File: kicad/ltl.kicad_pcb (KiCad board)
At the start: 2 copper layers, 73 x 46 mm, 14 parts, among them J1 Serial Connection, J2 BARREL_JACK, SW1 SW_DIP_x02, SW2 SW_DIP_x02, U1 ESP-12E, U2 DS18B20

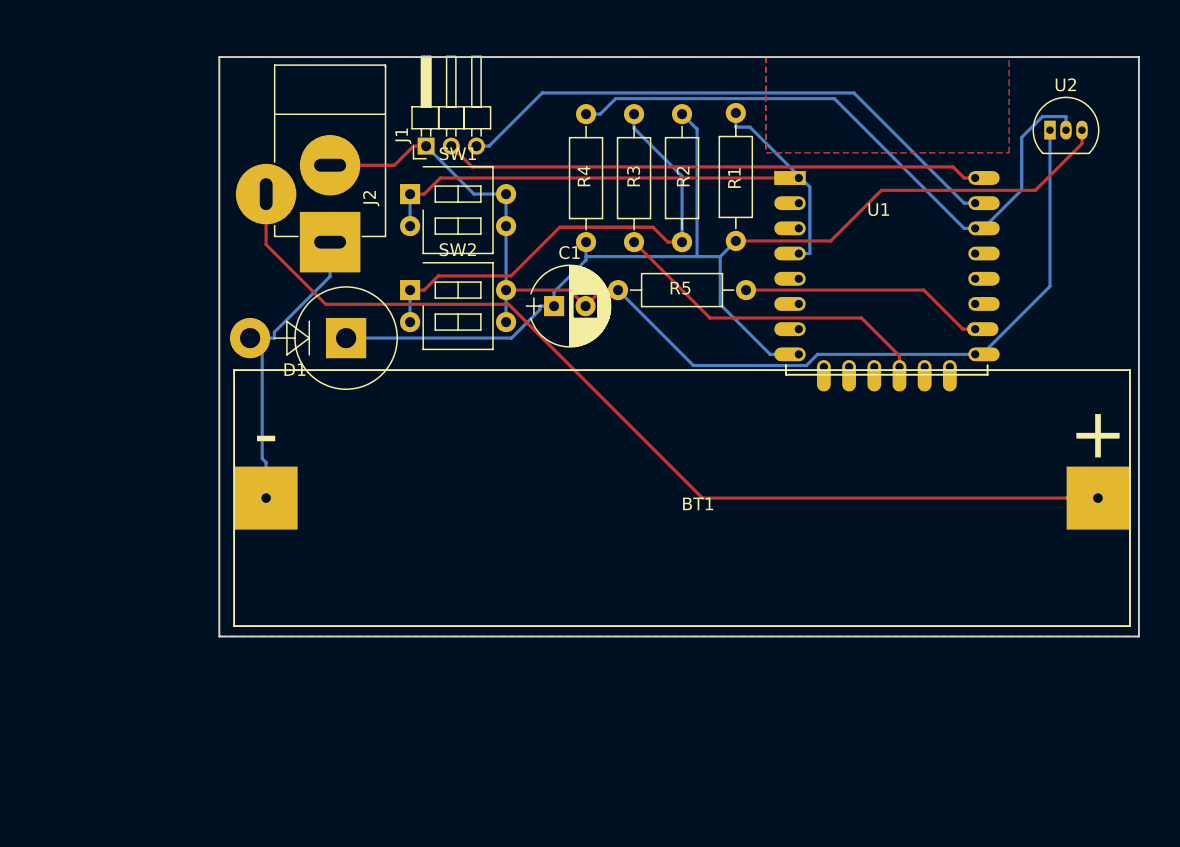
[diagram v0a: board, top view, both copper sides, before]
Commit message: letzte Änderungen
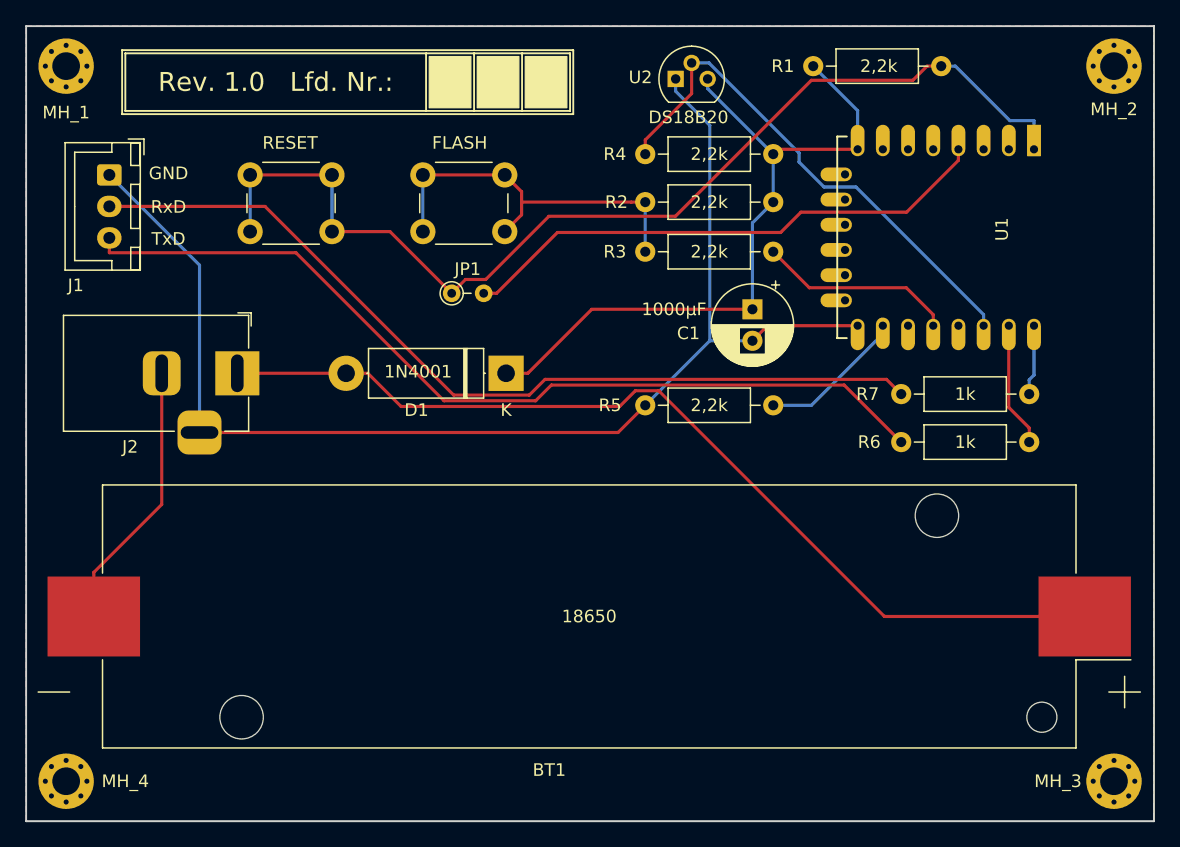
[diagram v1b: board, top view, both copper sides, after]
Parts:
- removed SW1, SW2: SW_DIP_x02, Buttons_Switches_THT:SW_DIP_x2_W7.62mm_Slide_LowProfile
- added FLASH: SW_DIP_x02, Button_Switch_THT:SW_PUSH_6mm_H5mm, F.Cu at (105.2, 79.8)
- added JP1: Jumper, Resistor_THT:R_Axial_DIN0204_L3.6mm_D1.6mm_P2.54mm_Vertical, F.Cu at (107.4, 89.2)
- added MH_1: MH_1, MountingHole:MountingHole_2.2mm_M2_Pad_Via, F.Cu at (76.8, 71.1)
- added MH_2: MH_2, MountingHole:MountingHole_2.2mm_M2_Pad_Via, F.Cu at (160.0, 71.1)
- added MH_3: MH_3, MountingHole:MountingHole_2.2mm_M2_Pad_Via, F.Cu at (160.0, 127.9)
- added MH_4: MH_4, MountingHole:MountingHole_2.2mm_M2_Pad_Via, F.Cu at (76.8, 127.9)
- added R6: 1k, Resistor_THT:R_Axial_DIN0207_L6.3mm_D2.5mm_P10.16mm_Horizontal, F.Cu at (143.1, 101.0)
- added R7: 1k, Resistor_THT:R_Axial_DIN0207_L6.3mm_D2.5mm_P10.16mm_Horizontal, F.Cu at (143.1, 97.2)
- added RESET: SW_DIP_x02, Button_Switch_THT:SW_PUSH_6mm_H5mm, F.Cu at (91.4, 79.8)
- BT1: footprint 18650:18650 -> Battery:BatteryHolder_Keystone_1042_1x18650
- C1: footprint Capacitors_THT:CP_Radial_D6.3mm_P2.50mm -> Capacitor_THT:CP_Radial_D6.3mm_P2.50mm
- D1: value D -> 1N4001; footprint Diodes_THT:D_5KPW_P7.62mm_Vertical_AnodeUp -> Diode_THT:D_5W_P12.70mm_Horizontal
- J1: value Serial Connection -> CONN_01X03; footprint Pin_Headers:Pin_Header_Angled_1x03_Pitch2.00mm -> Connector_JST:JST_XH_B3B-XH-A_1x03_P2.50mm_Vertical
- J2: footprint Connectors:JACK_ALIM -> Connector_BarrelJack:BarrelJack_Horizontal
- R1, R2, R3, R4, R5: footprint Resistors_THT:R_Axial_DIN0207_L6.3mm_D2.5mm_P10.16mm_Horizontal -> Resistor_THT:R_Axial_DIN0207_L6.3mm_D2.5mm_P10.16mm_Horizontal
- U2: footprint TO_SOT_Packages_THT:TO-92_Inline_Narrow_Oval -> Package_TO_SOT_THT:TO-92
- moved U2 30.0 mm to (125.2, 72.1)
- moved J1 25.2 mm to (80.3, 79.8), turned to 270 degrees
- moved U1 18.8 mm to (153.7, 77.7), turned to 270 degrees
- moved R4 16.4 mm to (133.0, 78.1), turned to 180 degrees
- moved C1 15.8 mm to (131.3, 90.4), turned to 270 degrees
- moved R1 15.2 mm to (136.1, 71.1), turned to 0 degrees
- moved D1 13.0 mm to (111.8, 95.5)
- moved BT1 12.8 mm to (118.4, 114.8), turned to 180 degrees
- moved J2 12.8 mm to (90.4, 95.5), turned to 0 degrees
- moved R3 11.1 mm to (133.0, 85.9), turned to 180 degrees
- moved R2 10.1 mm to (133.0, 81.9), turned to 180 degrees
- moved R5 9.40 mm to (122.8, 98.0)
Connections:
- J2 pad 2: GND -> Net-(BT1-Pad2)
- J2 pad 3: Net-(BT1-Pad2) -> GND
- R1 pad 2: Net-(R1-Pad2) -> Net-(JP1-Pad1)
- U1 pad 1: Net-(R1-Pad2) -> Net-(JP1-Pad1)
- U1 pad 12: Net-(U1-Pad12) -> Net-(R3-Pad1)
- U1 pad 15: /TxD -> Net-(R6-Pad2)
- U1 pad 16: /RxD -> Net-(R7-Pad2)
- U1 pad 20: Net-(R3-Pad1) -> Net-(U1-Pad20)
- U1 pad 4: Net-(R1-Pad2) -> Net-(JP1-Pad2)
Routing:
- net Net-(JP1-Pad1): track 0.00 -> 84.8 mm
- net Net-(BT1-Pad2): track 78.4 -> 21.5 mm
- net Net-(BT1-Pad1): track 24.2 -> 76.3 mm
- net Net-(R1-Pad2): track 49.2 -> 0.00 mm
- net Net-(JP1-Pad2): track 0.00 -> 42.9 mm
- net +3V3: track 91.5 -> 57.7 mm
- net /RxD: track 42.6 -> 70.1 mm
- net /TxD: track 45.0 -> 71.3 mm
- net GND: track 88.1 -> 101.1 mm
- net Net-(R3-Pad1): track 25.7 -> 15.6 mm
- net Net-(R6-Pad2): track 0.00 -> 9.91 mm
- net Net-(R4-Pad2): track 50.1 -> 41.5 mm
- net Net-(R2-Pad2): track 38.4 -> 30.4 mm
- net Net-(R5-Pad2): track 19.5 -> 11.7 mm
- net Net-(R7-Pad2): track 0.00 -> 5.59 mm
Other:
- board size 73 x 46 mm -> 89.5 x 63.1 mm
- board text added: "GND"
- board text added: "Rev. 1.0 Lfd. Nr.:"
- board text added: "RxD"
- board text added: "TxD"
